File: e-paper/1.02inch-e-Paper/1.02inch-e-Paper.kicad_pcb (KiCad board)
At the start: 2 copper layers, 40 x 20.9 mm, 23 parts, among them J1 Conn_01x06_Pin, J2 Conn_01x03_Pin

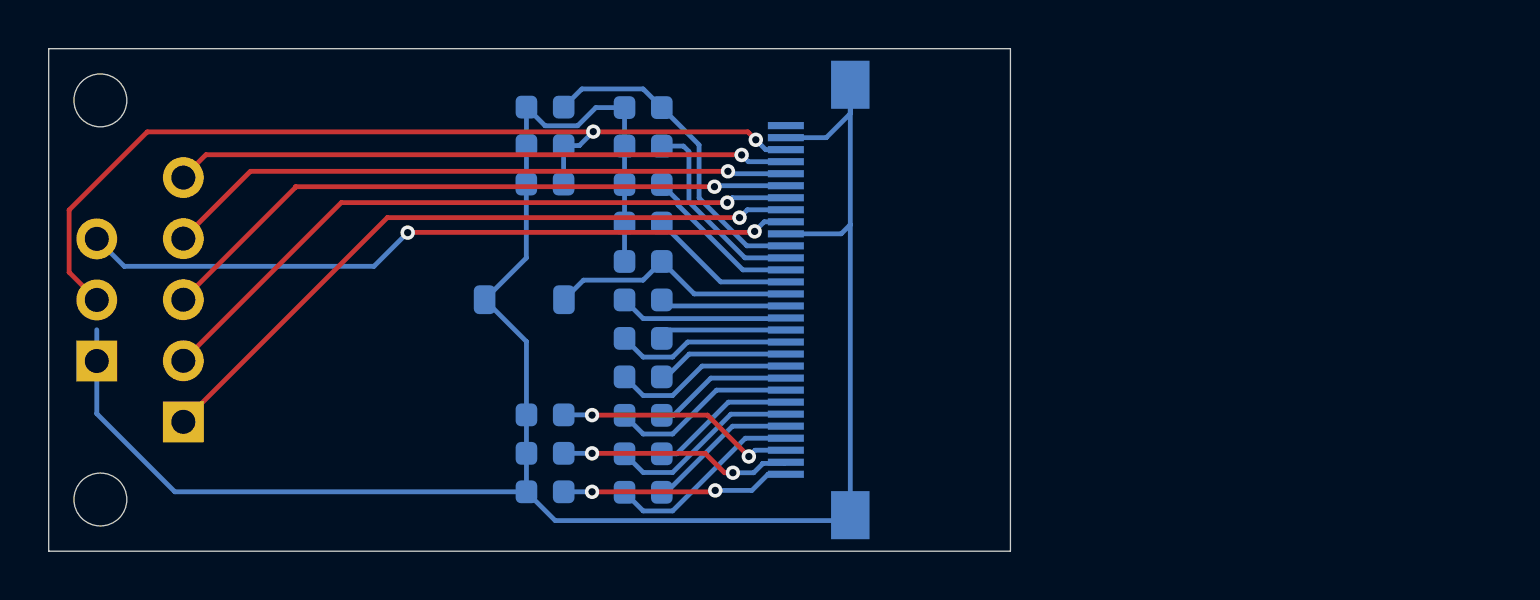
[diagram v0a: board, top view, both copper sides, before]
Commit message: update e-paper
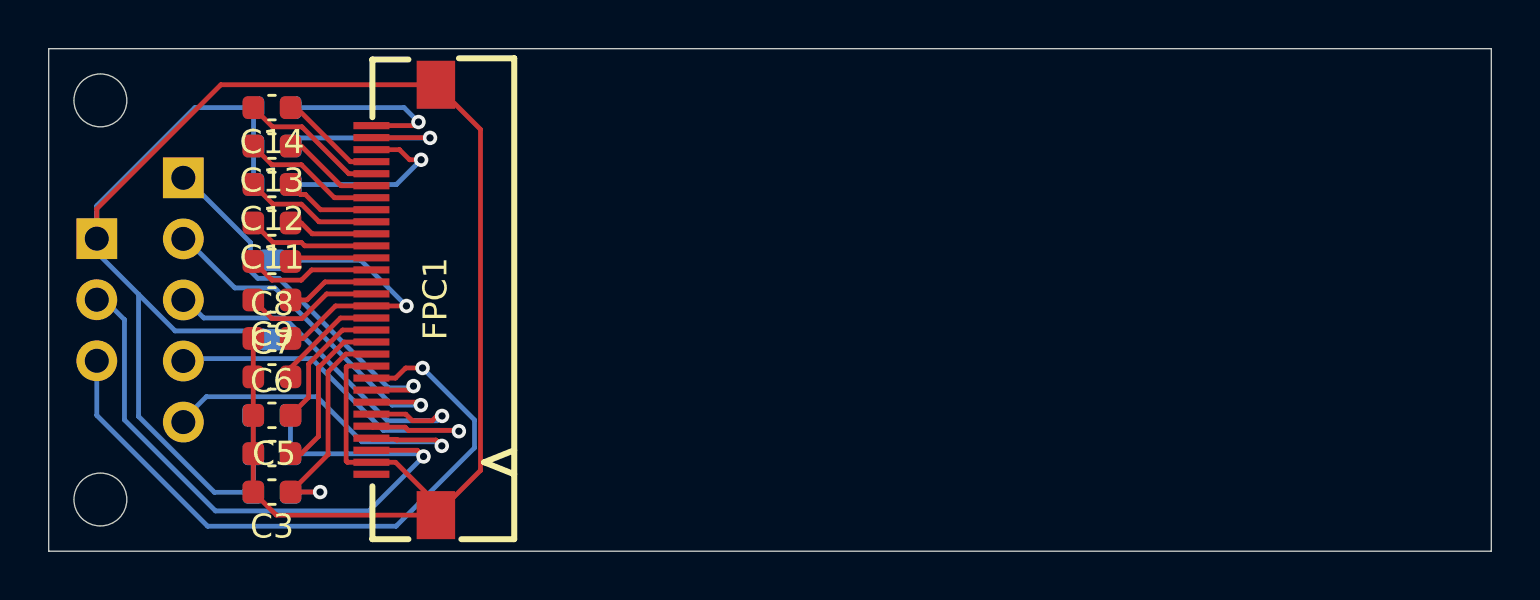
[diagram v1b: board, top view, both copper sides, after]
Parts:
- C10, C11, C12, C13, C14, C3, C5, C6, C7, C8, C9, FPC1: moved to F.Cu
- moved C14 22.2 mm to (9.29, -8.00), turned to 180 degrees
- moved C3 22.2 mm to (9.29, 7.99)
- moved C13 20.1 mm to (9.29, -6.40), turned to 180 degrees
- moved C5 20.0 mm to (9.29, 6.39)
- moved C4 19.6 mm to (9.29, 8.00)
- moved C17 19.6 mm to (9.29, -8.00)
- moved C12 18.2 mm to (9.29, -4.80), turned to 180 degrees
- moved C6 18.2 mm to (9.29, 4.80)
- moved FPC1 17.2 mm to (14.8, 0.00), turned to 90 degrees
- moved C1 17.1 mm to (9.29, 6.40)
- moved C16 17.1 mm to (9.29, -6.40)
- moved C11 16.7 mm to (9.29, -3.20), turned to 180 degrees
- moved C7 16.7 mm to (9.29, 3.20)
- moved C10 15.8 mm to (9.29, -1.60), turned to 180 degrees
- moved C8 15.8 mm to (9.29, 1.60)
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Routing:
- net DC: track 27.9 -> 14.9 mm
- net RST: track 28.7 -> 15.8 mm
- net CS: track 27.0 -> 16.1 mm
- net DIN: track 25.6 -> 15.1 mm
- net CLK: track 26.3 -> 16.4 mm
- net 3.3V: track 38.8 -> 30.3 mm, vias 2 -> 1
- net GND: track 90.4 -> 98.1 mm
- net Net-(C14-Pad1): track 8.28 -> 4.29 mm
- net Net-(C13-Pad1): track 8.04 -> 4.05 mm
- net Net-(C12-Pad1): track 7.79 -> 3.80 mm
- net Net-(C11-Pad1): track 7.54 -> 3.60 mm
- net Net-(C10-Pad1): track 7.29 -> 3.42 mm
- net Net-(C9-Pad1): track 7.04 -> 3.67 mm
- net Net-(C3-Pad1): track 13.6 -> 10.2 mm, vias 0 -> 1
- net Net-(C15-Pad2): track 10.1 -> 8.09 mm, vias 2 -> 1
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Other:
- board size 40 x 20.9 mm -> 60 x 20.9 mm
